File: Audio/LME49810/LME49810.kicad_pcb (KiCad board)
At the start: 2 copper layers, 81.3 x 94 mm, 31 parts, among them Q1 NPN(TO-3P-BCE), Q2 PNP(TO-3P-BCE), Q3 NPN(TO-220-BCE), U1 LME49810

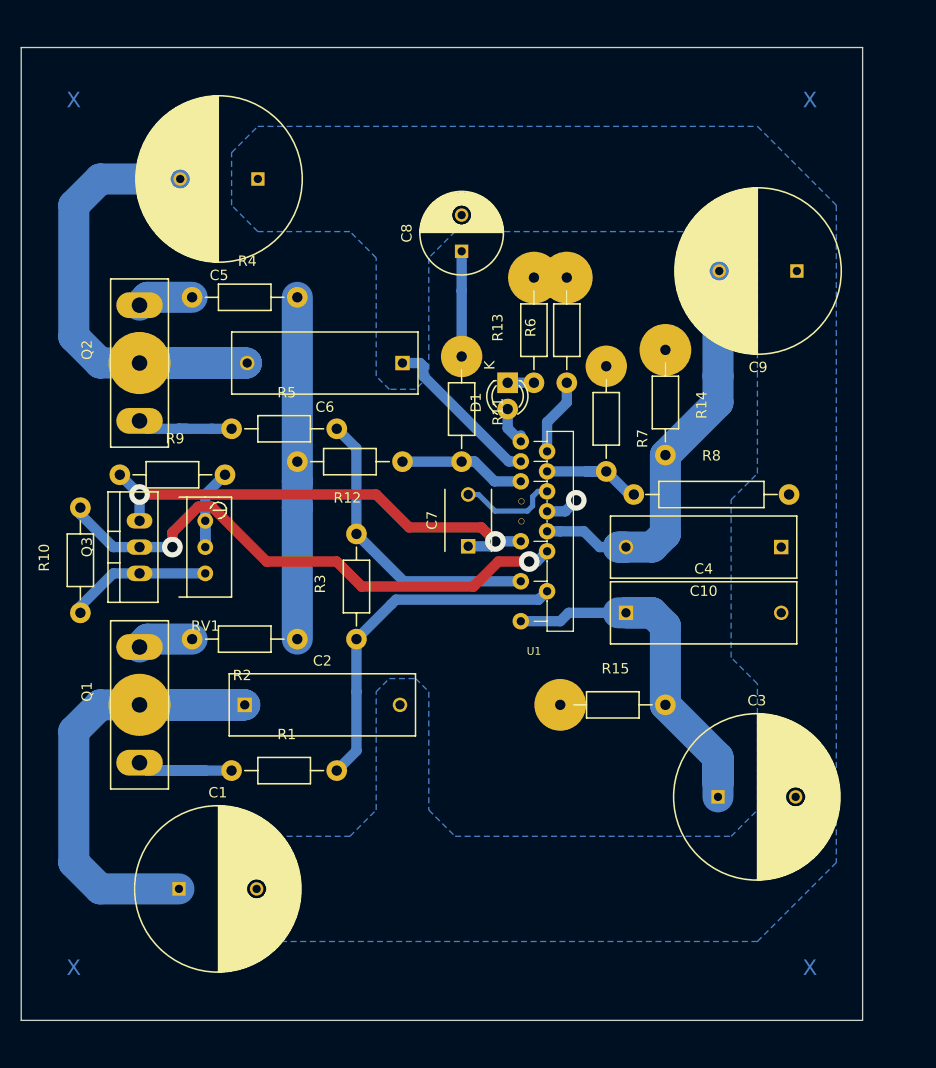
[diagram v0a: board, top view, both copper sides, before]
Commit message: Fixes
More fixes done
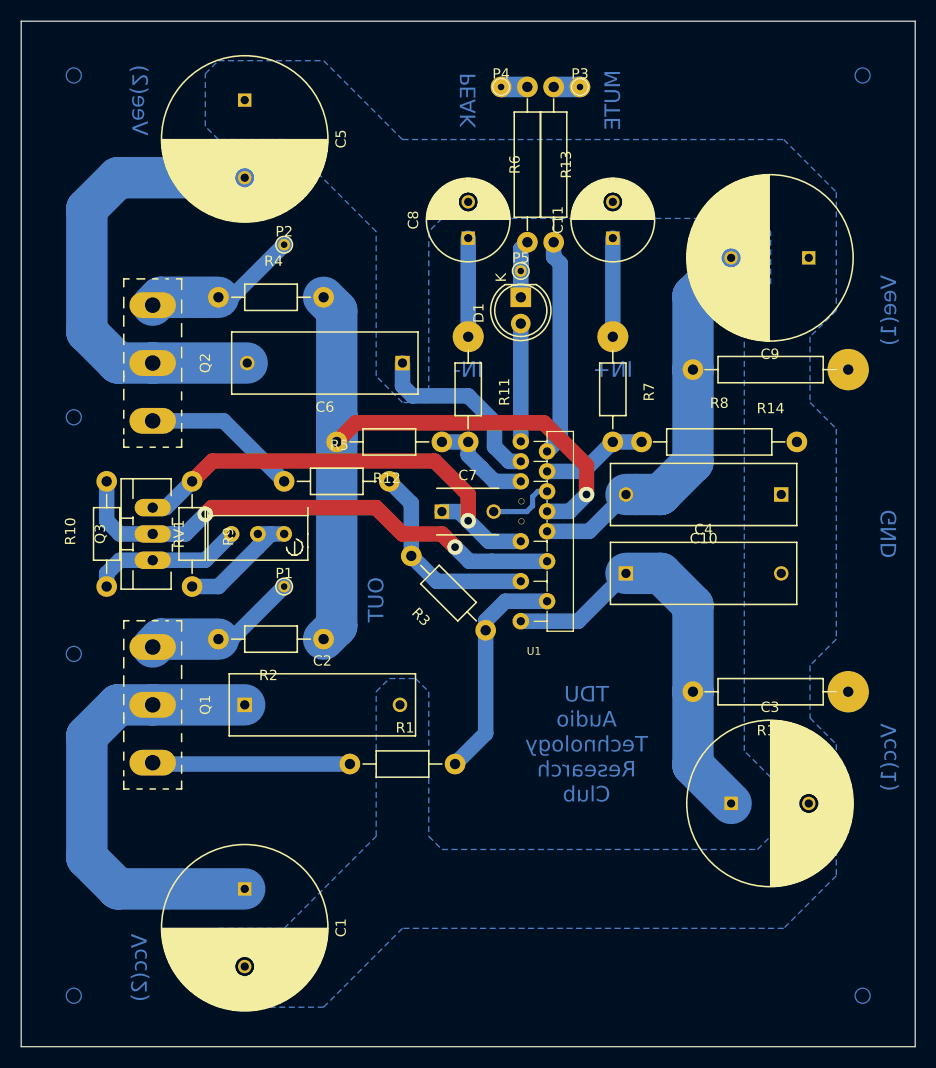
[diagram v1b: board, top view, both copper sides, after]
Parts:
- added C11: 470u, Capacitors_ThroughHole:C_Radial_D8_L11.5_P3.5, F.Cu at (82.5, 43.8)
- added P1: CONN_01X01, Connect:PINTST, F.Cu at (50.8, 77.5)
- added P2: CONN_01X01, Connect:PINTST, F.Cu at (50.8, 44.5)
- added P3: CONN_01X01, Connect:PINTST, F.Cu at (79.4, 29.2)
- added P4: CONN_01X01, Connect:PINTST, F.Cu at (71.8, 29.2)
- added P5: CONN_01X01, Connect:PINTST, F.Cu at (73.7, 47.0)
- D1: footprint LEDs:LED-3MM -> LEDs:LED-5MM
- Q1, Q2: footprint Transistors_TO-247:TO-247_Vertical_Neutral123 -> TO_SOT_Packages_THT:TO-247_Vertical_Neutral123_MountedFromLS
- Q3: footprint Transistors_TO-220:TO-220_Neutral123_Vertical -> TO_SOT_Packages_THT:TO-220_Neutral123_Vertical_LargePads
- R11, R7: value 240 -> 470
- R12, R8: value 6.8k -> 7.5k
- R13, R14, R15, R6: footprint Resistors_ThroughHole:Resistor_Horizontal_RM10mm -> Resistors_ThroughHole:Resistor_Horizontal_RM15mm
- R9: value 360 -> 330
- RV1: value 200 -> 500
- moved R6 16.0 mm to (76.8, 36.7)
- moved R13 16.0 mm to (74.3, 36.7), turned to 270 degrees
- moved R15 15.3 mm to (97.8, 87.6), turned to 180 degrees
- moved R1 11.4 mm to (62.2, 94.6)
- moved R14 10.6 mm to (97.8, 56.5), turned to 180 degrees
- moved R3 8.91 mm to (66.7, 78.1), turned to 135 degrees
- moved D1 8.35 mm to (73.7, 49.5)
- moved C5 7.73 mm to (47.0, 30.5), turned to 270 degrees
- moved RV1 7.73 mm to (50.8, 72.4), turned to 90 degrees
- moved R5 7.18 mm to (55.9, 67.3)
- moved C1 6.35 mm to (47.0, 106.7), turned to 270 degrees
- moved R9 6.02 mm to (41.9, 72.4), turned to 270 degrees
- moved R8 5.14 mm to (92.8, 63.5)
- moved C10 5.08 mm to (98.8, 68.6)
- moved R12 4.26 mm to (61.0, 63.5)
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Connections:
- net Net-(C10-Pad2) renamed /Vee
- net Net-(C3-Pad1) renamed /Vcc
- net Net-(C8-Pad1) renamed /IN-
- net Net-(Q1-Pad3) renamed /Emit-NPN
- net Net-(Q2-Pad3) renamed /Emit-PNP
- R13 pad 1: Net-(D1-Pad1) -> Net-(P4-Pad1)
- R13 pad 2: +5V -> Net-(D1-Pad1)
- R14 pad 1: -VeeL1 -> (no net)
- R15 pad 1: +VccL1 -> (no net)
- R6 pad 2: +5V -> Net-(P3-Pad1)
- R7 pad 1: /InputLH -> /IN+
- U1 pad 7: Net-(U1-Pad7) -> (no net)
- U1 pad 9: Net-(U1-Pad9) -> (no net)
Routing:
- net OUTLH: track 41.4 -> 70.5 mm
- net -VeeL2: track 63.7 -> 45.1 mm
- net +VccL2: track 63.1 -> 44.8 mm
- net Net-(R6-Pad1): track 7.42 -> 21.0 mm
- net SourceLH: track 33.8 -> 21.8 mm
- net /Emit-PNP: track 5.40 -> 15.1 mm
- net /Emit-NPN: track 5.40 -> 15.1 mm
- net /IN+: track 0.00 -> 9.53 mm
- net SinkLH: track 28.8 -> 19.7 mm
- net Net-(D1-Pad2): track 4.16 -> 11.4 mm
- net Net-(Q2-Pad1): track 10.7 -> 15.1 mm
- net CLH: track 54.1 -> 50.1 mm
- net Net-(D1-Pad1): track 3.18 -> 6.85 mm
- net Net-(R11-Pad2): track 13.5 -> 9.94 mm
- net Net-(C7-Pad2): track 9.77 -> 6.49 mm
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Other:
- board size 81.3 x 94 mm -> 86.4 x 99.1 mm
- net class Default: trace_width 1 -> 1.5; via_dia 2 -> 1.5; via_drill 1 -> 0.75
- net class Thick: trace_width 3 -> 4
- board text added: "GND"
- board text added: "IN+"
- board text added: "IN-"
- board text added: "MUTE"
- board text added: "OUT"
- board text added: "PEAK"
- board text added: "TDU Audio Technology Research Club"
- board text added: "Vcc(1)"
- board text added: "Vcc(2)"
- board text added: "Vee(1)"
- board text added: "Vee(2)"
- board text added: "○"
- board text removed: "X"
